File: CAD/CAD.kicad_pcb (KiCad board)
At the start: 2 copper layers, 132.1 x 86.4 mm, 11 parts, among them M1 Motor_Servo_Hitec, SW1 SW_Push, U1 RFID_RC522, U2 LCD_1602_I2C

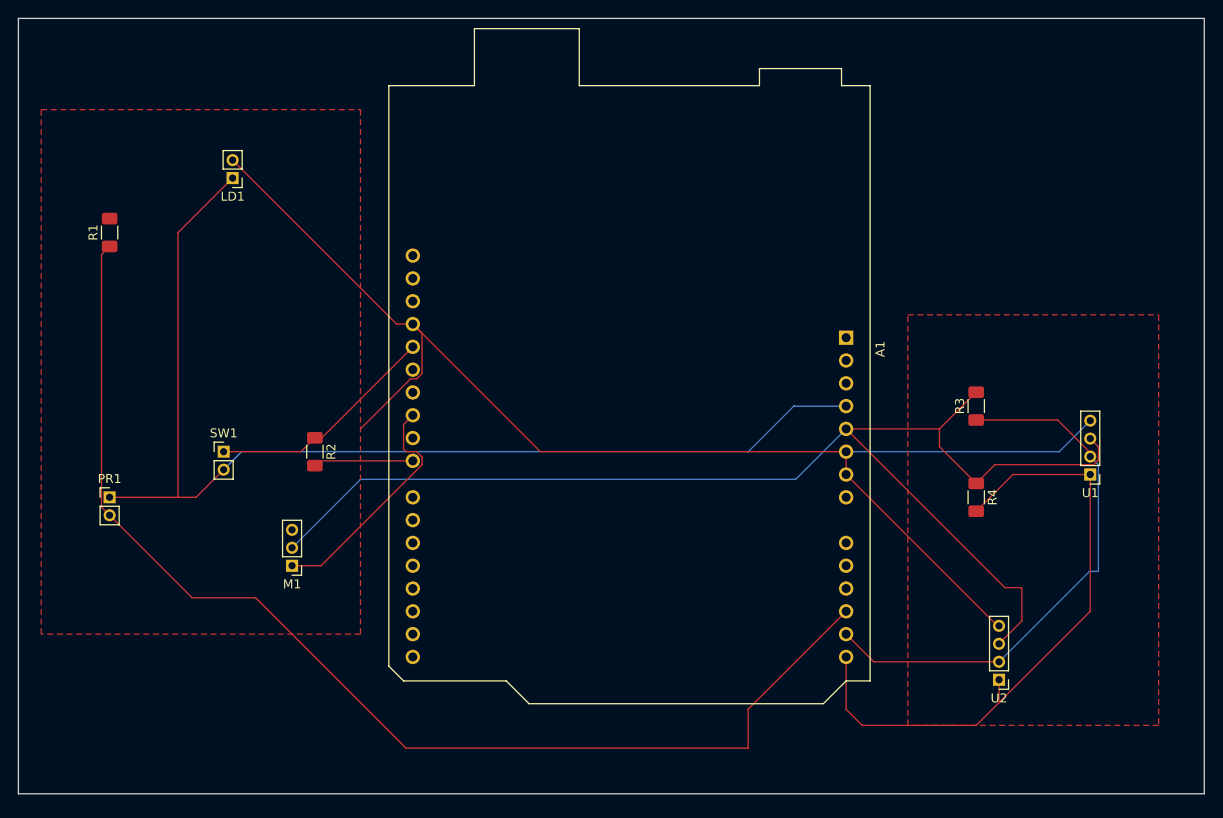
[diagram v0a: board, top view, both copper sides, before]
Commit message: Final CAD
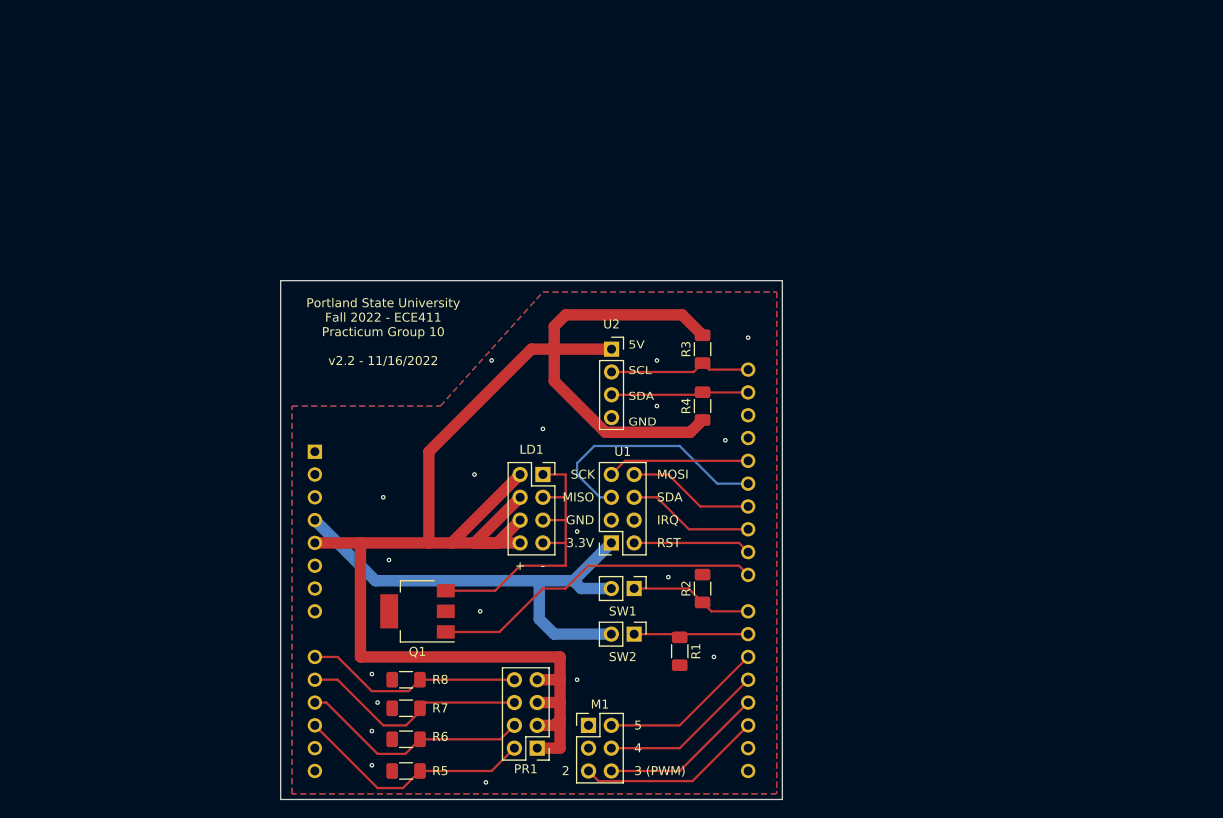
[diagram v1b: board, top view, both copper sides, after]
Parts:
- added Q1: 2N7002, Package_TO_SOT_SMD:SOT-223-3_TabPin2, F.Cu at (118.1, 96.5)
- added R5: 10k, Resistor_SMD:R_1206_3216Metric_Pad1.30x1.75mm_HandSolder, F.Cu at (116.8, 114.3)
- added R6: 10k, Resistor_SMD:R_1206_3216Metric_Pad1.30x1.75mm_HandSolder, F.Cu at (116.8, 110.8)
- added R7: 10k, Resistor_SMD:R_1206_3216Metric_Pad1.30x1.75mm_HandSolder, F.Cu at (116.8, 107.3)
- added R8: 10k, Resistor_SMD:R_1206_3216Metric_Pad1.30x1.75mm_HandSolder, F.Cu at (116.8, 104.1)
- added SW2: SW_Push, Connector_PinHeader_2.54mm:PinHeader_1x02_P2.54mm_Vertical, F.Cu at (142.2, 99.1)
- A1: moved to B.Cu
- LD1: footprint Connector_PinHeader_2.00mm:PinHeader_1x02_P2.00mm_Vertical -> Connector_PinSocket_2.54mm:PinSocket_2x04_P2.54mm_Vertical
- M1: footprint Connector_PinHeader_2.00mm:PinHeader_1x03_P2.00mm_Vertical -> Connector_PinHeader_2.54mm:PinHeader_2x03_P2.54mm_Vertical
- PR1: footprint Connector_PinHeader_2.00mm:PinHeader_1x02_P2.00mm_Vertical -> Connector_PinHeader_2.54mm:PinHeader_2x04_P2.54mm_Vertical
- R1: value 100 -> 10k
- SW1: footprint Connector_PinHeader_2.00mm:PinHeader_1x02_P2.00mm_Vertical -> Connector_PinHeader_2.54mm:PinHeader_1x02_P2.54mm_Vertical
- U1: footprint Connector_PinHeader_2.00mm:PinHeader_1x04_P2.00mm_Vertical -> Connector_PinSocket_2.54mm:PinSocket_2x04_P2.54mm_Vertical
- U2: footprint Connector_PinHeader_2.00mm:PinHeader_1x04_P2.00mm_Vertical -> Connector_PinSocket_2.54mm:PinSocket_1x04_P2.54mm_Vertical
- moved R1 78.8 mm to (147.3, 101.0), turned to -90 degrees
- moved A1 60.5 mm to (106.7, 78.7)
- moved U2 56.7 mm to (139.7, 67.3), turned to 0 degrees
- moved PR1 55.2 mm to (131.4, 111.8), turned to 180 degrees
- moved U1 53.9 mm to (139.7, 88.9)
- moved SW1 48.2 mm to (142.2, 94.0), turned to -90 degrees
- moved LD1 47.8 mm to (132.1, 81.3), turned to 0 degrees
- moved R2 45.8 mm to (149.9, 94.0), turned to 90 degrees
- moved M1 37.5 mm to (137.2, 109.2), turned to 0 degrees
- moved R4 32.1 mm to (149.9, 73.7), turned to 90 degrees
- moved R3 31.1 mm to (149.9, 67.3)
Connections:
- A1 pad 10: unconnected-(A1-Pad10) -> Net-(A1-Pad10)
- A1 pad 11: unconnected-(A1-Pad11) -> Net-(A1-Pad11)
- A1 pad 13: Net-(A1-Pad13) -> unconnected-(A1-Pad13)
- A1 pad 14: Net-(A1-Pad14) -> unconnected-(A1-Pad14)
- A1 pad 17: unconnected-(A1-Pad17) -> Net-(A1-Pad17)
- A1 pad 18: unconnected-(A1-Pad18) -> Net-(A1-Pad18)
- A1 pad 19: unconnected-(A1-Pad19) -> Net-(A1-Pad19)
- A1 pad 20: unconnected-(A1-Pad20) -> Net-(A1-Pad20)
- A1 pad 21: unconnected-(A1-Pad21) -> Net-(A1-Pad21)
- A1 pad 22: unconnected-(A1-Pad22) -> Net-(A1-Pad22)
- A1 pad 23: GND -> Net-(A1-Pad23)
- A1 pad 24: unconnected-(A1-Pad24) -> Net-(A1-Pad24)
- A1 pad 26: unconnected-(A1-Pad26) -> Net-(A1-Pad26)
- A1 pad 27: unconnected-(A1-Pad27) -> Net-(A1-Pad27)
- A1 pad 31: unconnected-(A1-Pad31) -> Net-(A1-Pad31)
- A1 pad 32: unconnected-(A1-Pad32) -> Net-(A1-Pad32)
- A1 pad 9: unconnected-(A1-Pad9) -> Net-(A1-Pad9)
- LD1 pad 1: +3.3V -> Net-(LD1-Pad1)
- LD1 pad 2: GND -> +5V
- M1 pad 1: Net-(A1-Pad25) -> +9V
- M1 pad 2: +5V -> Net-(A1-Pad20)
- PR1 pad 1: +3.3V -> +5V
- R1 pad 1: Net-(A1-Pad12) -> Net-(A1-Pad21)
- R2 pad 1: Net-(A1-Pad28) -> Net-(A1-Pad22)
- R3 pad 1: Net-(A1-Pad13) -> Net-(A1-Pad32)
- R4 pad 2: Net-(A1-Pad14) -> Net-(A1-Pad31)
- SW1 pad 1: Net-(A1-Pad28) -> Net-(A1-Pad22)
- U1 pad 1: Net-(A1-Pad14) -> +3.3V
- U1 pad 2: Net-(A1-Pad13) -> Net-(A1-Pad24)
- U1 pad 3: +5V -> (no net)
- U1 pad 4: GND -> unconnected-(U1-Pad4)
- U2 pad 1: Net-(A1-Pad14) -> +5V
- U2 pad 2: Net-(A1-Pad13) -> Net-(A1-Pad32)
- U2 pad 3: +5V -> Net-(A1-Pad31)
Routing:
- net GND: track 163.5 -> 0.00 mm, vias 0 -> 19
- net Net-(A1-Pad12): track 132.3 -> 27.0 mm
- net Net-(A1-Pad14): track 71.2 -> 0.00 mm
- net +3.3V: track 124.3 -> 55.1 mm
- net Net-(A1-Pad13): track 61.2 -> 0.00 mm
- net +5V: track 142.7 -> 181.2 mm
- net Net-(A1-Pad23): track 0.00 -> 37.2 mm
- net Net-(LD1-Pad1): track 0.00 -> 34.8 mm
- net Net-(A1-Pad27): track 0.00 -> 27.7 mm
- net Net-(A1-Pad11): track 0.00 -> 25.9 mm
- net Net-(A1-Pad10): track 0.00 -> 25.6 mm
- net Net-(A1-Pad9): track 0.00 -> 24.3 mm
- net Net-(A1-Pad17): track 0.00 -> 20.8 mm
- net Net-(A1-Pad20): track 0.00 -> 18.4 mm
- net Net-(A1-Pad19): track 0.00 -> 18.4 mm
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- added copper zone on B.Cu, net GND
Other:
- board size 132.1 x 86.4 mm -> 55.9 x 57.8 mm
- rule pad_to_mask_clearance: 0.0508 -> 0.1016
- board text added: "+"
- board text added: "-"
- board text added: "2"
- board text added: "3 (PWM)"
- board text added: "3.3V"
- board text added: "4"
- board text added: "5"
- board text added: "5V SCL SDA GND"
- board text added: "GND"
- board text added: "IRQ"
- board text added: "MISO"
- board text added: "MOSI"
- board text added: "Portland State University Fall 2022 - ECE411 Practicum Group 10 v2.2 - 11/16/2022"
- board text added: "RST"
- board text added: "SCK"
- board text added: "SDA"
